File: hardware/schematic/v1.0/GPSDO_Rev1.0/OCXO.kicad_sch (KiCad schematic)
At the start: 2 parts, among them U2 LMK1C1103PWR, U3 TMP117AIDRVR

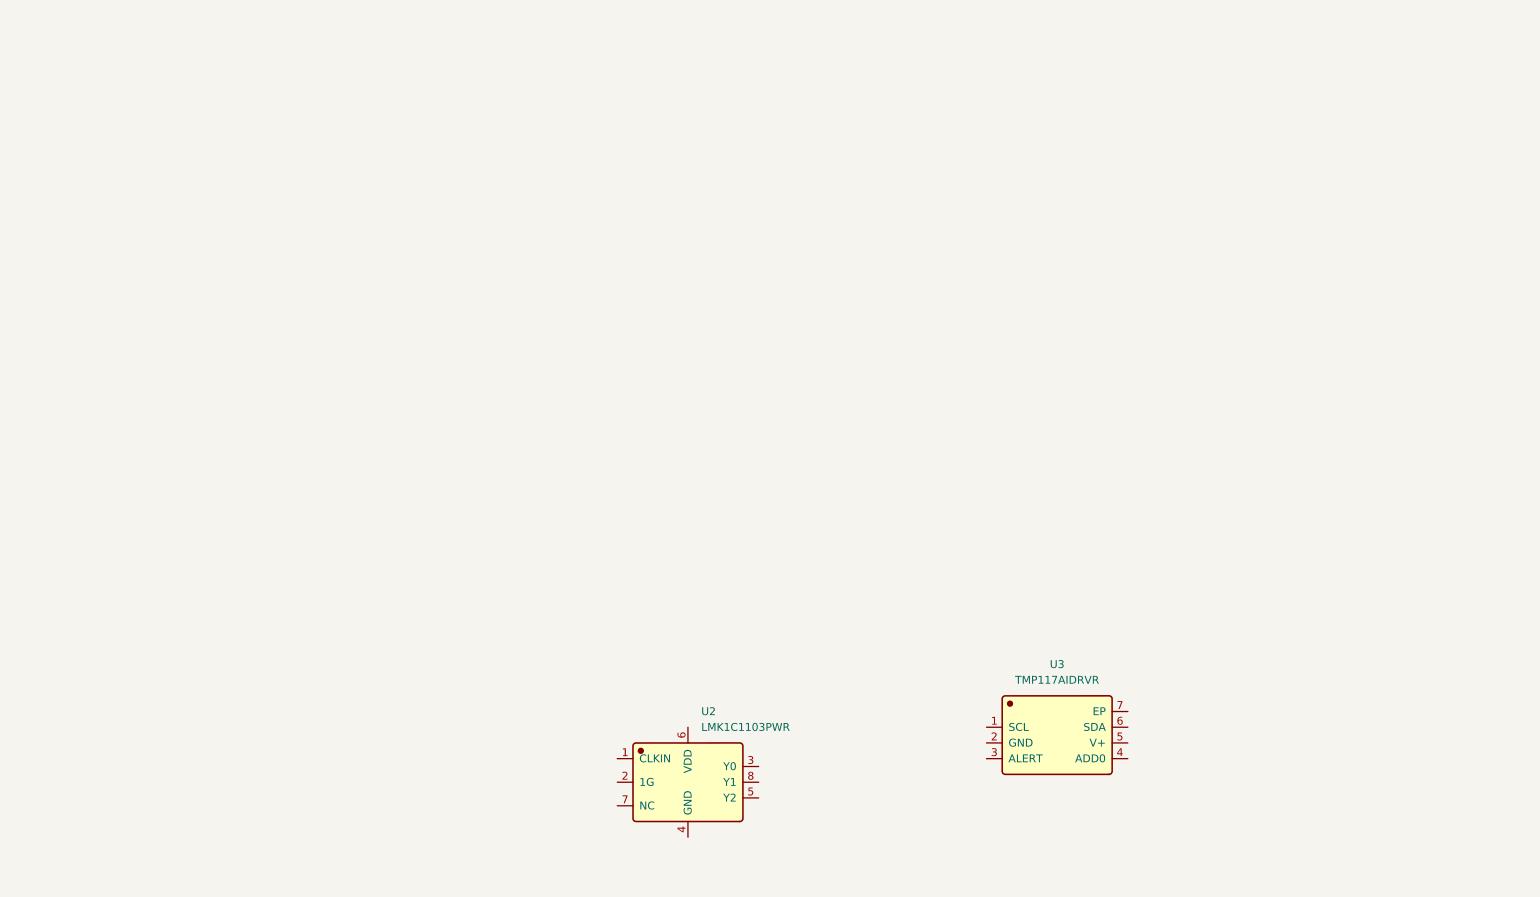
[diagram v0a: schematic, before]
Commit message: sch update
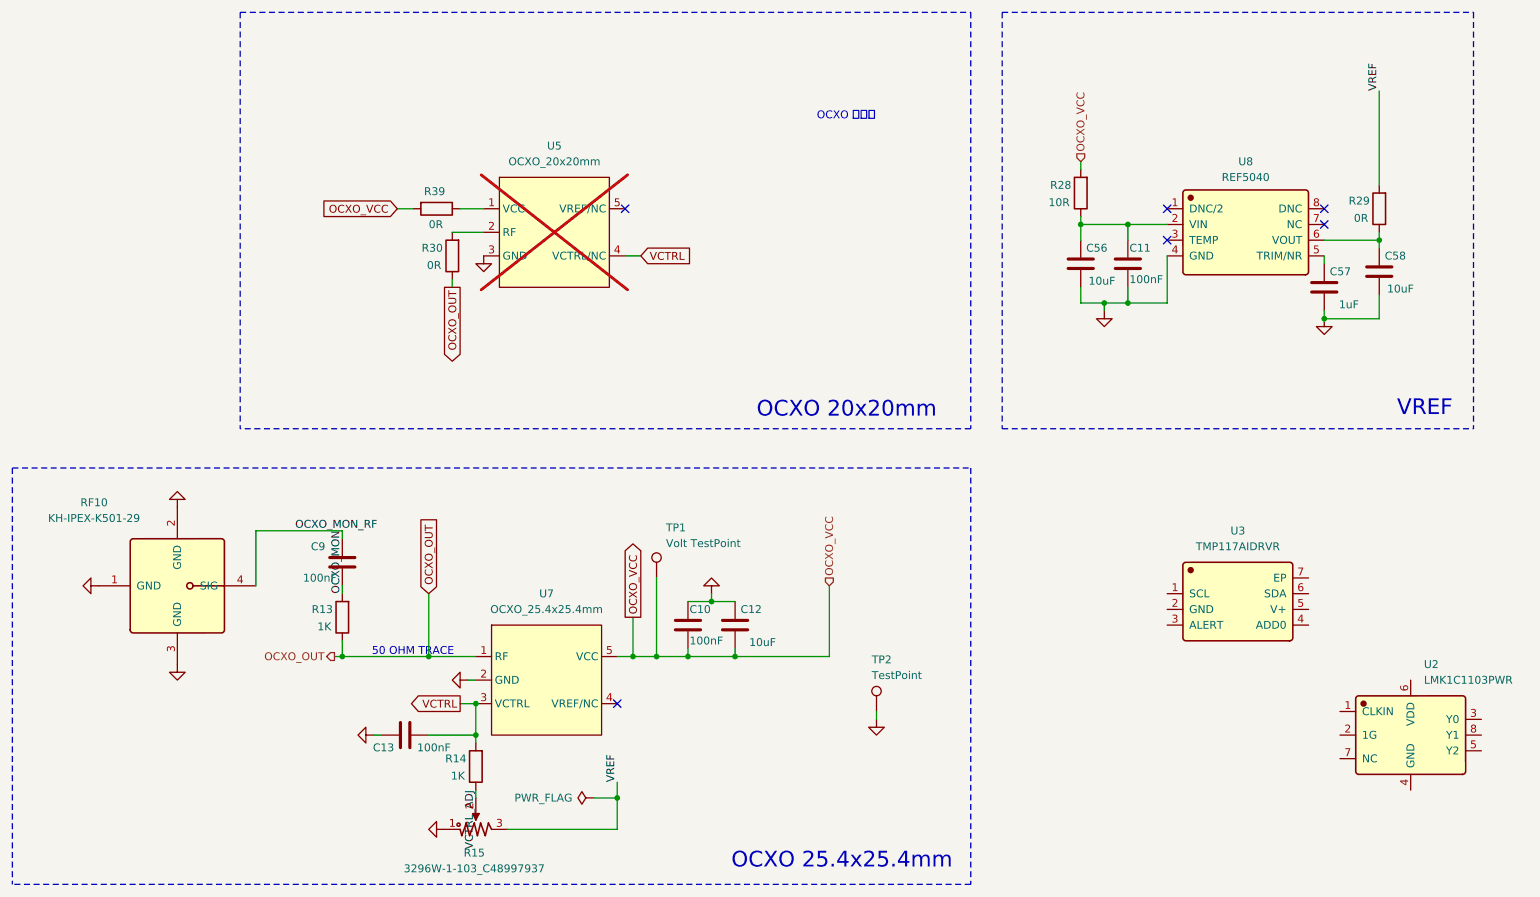
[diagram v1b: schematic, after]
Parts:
- added C10, C11, C13, C9: 100nF, Capacitor_SMD:C_0402_1005Metric, symbol Device:C
- added C12, C56, C58: 10uF, Capacitor_SMD:C_0603_1608Metric, symbol Device:C
- added C57: 1uF, Capacitor_SMD:C_0603_1608Metric, symbol Device:C
- added R13, R14: 1K, Resistor_SMD:R_0402_1005Metric, symbol Device:R
- added R15: 3296W-1-103_C48997937, Counter:3296W-1-103_C48997937, symbol Counter:3296W-1-103_C48997937
- added R28: 10R, Resistor_SMD:R_0603_1608Metric, symbol Device:R
- added R29: 0R, Resistor_SMD:R_0603_1608Metric, symbol Device:R
- added R30: 0R, Resistor_SMD:R_0402_1005Metric, symbol Device:R
- added R39: 0R, Resistor_SMD:R_0805_2012Metric, symbol Device:R
- added RF10: KH-IPEX-K501-29, JLCImport:KH-IPEX-K501-29, symbol JLCImport:KH-IPEX-K501-29
- added TP1: Volt TestPoint, TestPoint:TestPoint_Pad_D1.0mm, symbol Connector:TestPoint
- added TP2: TestPoint, TestPoint:TestPoint_Pad_D1.0mm, symbol Connector:TestPoint
- added U5: OCXO_20x20mm, JLCImport:OCXO_20x20mm, symbol Counter:OCXO_20x20mm
- added U7: OCXO_25.4x25.4mm, JLCImport:DOPFITKR2-10M, symbol Counter:OCXO_25.4x25.4mm
- added U8: REF5040, JLCImport:REF5040, symbol JLCImport:REF5040
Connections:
- new net: C11.2, C56.1, R28.1, U8.2 (VIN)
- new net: C57.1, U8.5 (TRIM/NR)
- new net: C58.1, R29.1, U8.6 (VOUT)
- new net: R30.2, U5.2 (RF)
- new net: R39.1, U5.1 (VCC)
- new net GND: C10.2, C11.1, C12.1, C13.2, C56.2, C57.2, C58.2, R15.1, RF10.1 (GND), RF10.2 (GND), RF10.3 (GND), TP2.1, U5.3 (GND), U7.2 (GND), U8.4 (GND)
- new net OCXO_MON: C9.2, R13.2
- new net OCXO_MON_RF: C9.1, RF10.4 (SIG)
- new net OCXO_OUT: R13.1, R30.1, U7.1 (RF)
- new net OCXO_VCC: C10.1, C12.2, R28.2, R39.2, TP1.1, U7.5 (VCC)
- new net VCTRL: C13.1, R14.2, U5.4 (VCTRL/NC), U7.3 (VCTRL)
- new net VCTRL_ADJ: R14.1, R15.2
- new net VREF: R15.3, R29.2
- no-connect marks 0 -> 6
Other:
- note added: "50 OHM TRACE"
- note added: "OCXO 20x20mm"
- note added: "OCXO 25.4x25.4mm"
- note added: "OCXO 二选一"
- note added: "VREF"
- moved on the sheet: U2, U3
